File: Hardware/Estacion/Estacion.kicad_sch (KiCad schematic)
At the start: 13 parts, among them J1 Screw_Terminal_01x02, J2 Step_Down_Mini

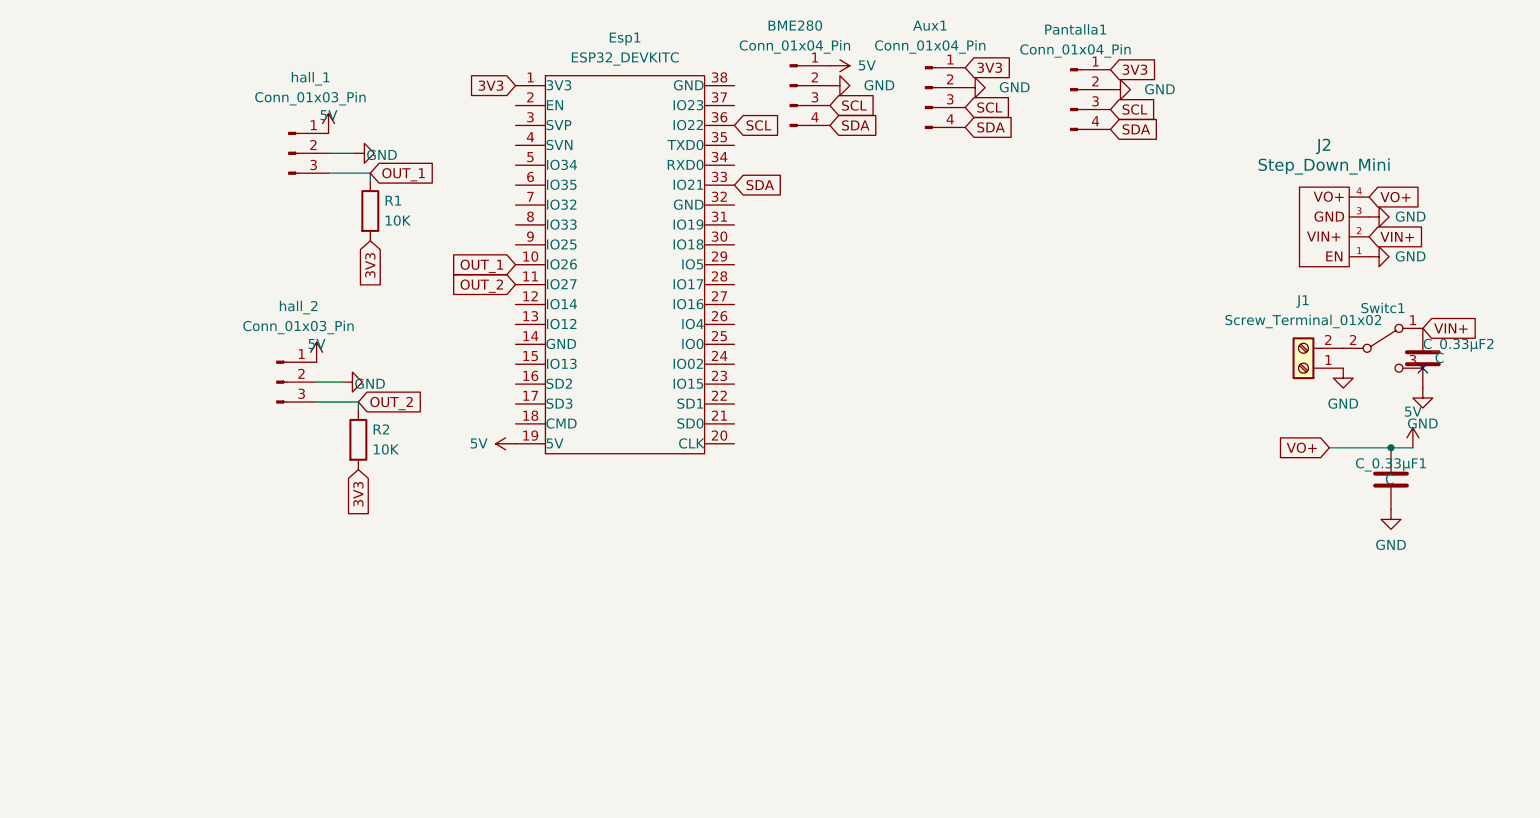
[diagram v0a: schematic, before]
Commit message: se avanzo el PCB y ESQUEMATICO
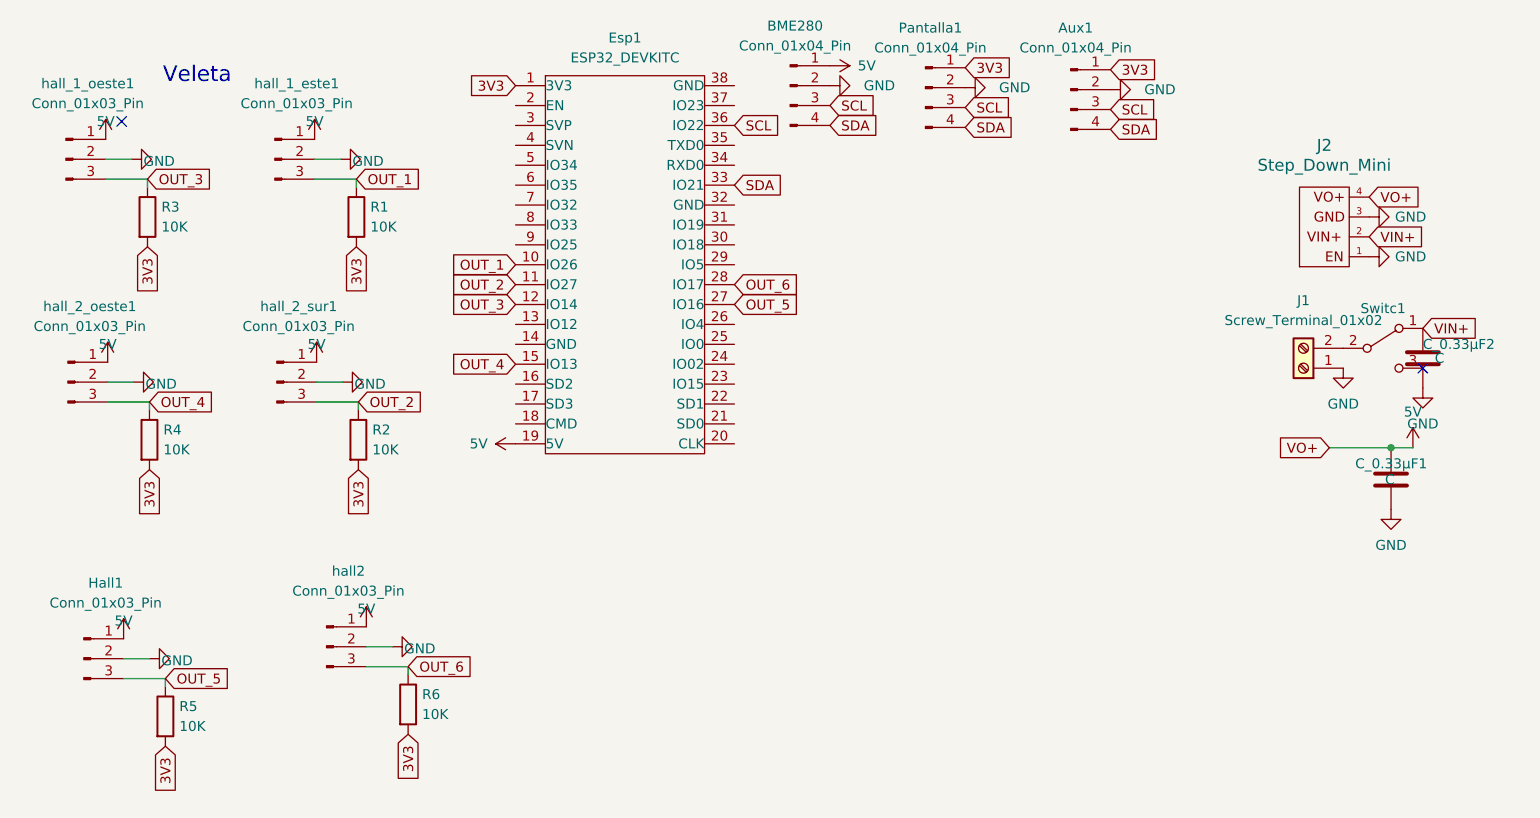
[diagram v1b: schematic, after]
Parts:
- added Hall1, hall2, hall_1_oeste1, hall_2_oeste1: Conn_01x03_Pin, Connector_JST:JST_PH_B3B-PH-K_1x03_P2.00mm_Vertical, symbol Connector:Conn_01x03_Pin
- added R3, R4, R5, R6: 10K, Resistor_SMD:R_0805_2012Metric_Pad1.20x1.40mm_HandSolder, symbol Device:R
- Aux1: renamed from Pantalla1; footprint Connector_PinSocket_2.54mm:PinSocket_1x04_P2.54mm_Vertical -> Connector_JST:JST_PH_B4B-PH-K_1x04_P2.00mm_Vertical
- BME280: footprint Connector_PinSocket_2.54mm:PinSocket_1x04_P2.54mm_Vertical -> Connector_JST:JST_PH_B4B-PH-K_1x04_P2.00mm_Vertical
- Pantalla1: renamed from Aux1; footprint Connector_PinSocket_2.54mm:PinSocket_1x04_P2.54mm_Vertical -> Connector_JST:JST_PH_B4B-PH-K_1x04_P2.00mm_Vertical
- R1, R2: footprint (none) -> Resistor_SMD:R_0805_2012Metric_Pad1.20x1.40mm_HandSolder
- hall_1_este1: renamed from hall_1; footprint Connector_PinHeader_2.54mm:PinHeader_1x03_P2.54mm_Vertical -> Connector_JST:JST_PH_B3B-PH-K_1x03_P2.00mm_Vertical
- hall_2_sur1: renamed from hall_2; footprint Connector_PinHeader_2.54mm:PinHeader_1x03_P2.54mm_Vertical -> Connector_JST:JST_PH_B3B-PH-K_1x03_P2.00mm_Vertical
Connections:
- net 3V3: now also R3.2, R4.2, R5.2, R6.2
- net 5V: now also Hall1.1 (Pin_1), hall2.1 (Pin_1), hall_1_oeste1.1 (Pin_1), hall_2_oeste1.1 (Pin_1)
- net GND: now also Hall1.2 (Pin_2), hall2.2 (Pin_2), hall_1_oeste1.2 (Pin_2), hall_2_oeste1.2 (Pin_2)
- net OUT_3: now reaches Esp1.12 (IO14)
- net OUT_3: now also R3.1, hall_1_oeste1.3 (Pin_3)
- net OUT_4: now reaches Esp1.15 (IO13)
- net OUT_4: now also R4.1, hall_2_oeste1.3 (Pin_3)
- net OUT_5: now reaches Esp1.27 (IO16)
- net OUT_5: now also Hall1.3 (Pin_3), R5.1
- net OUT_6: now reaches Esp1.28 (IO17)
- net OUT_6: now also R6.1, hall2.3 (Pin_3)
- no-connect marks 1 -> 2
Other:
- note added: "Veleta"
- moved on the sheet: R1, hall_1_este1

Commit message: Primera version del PCB
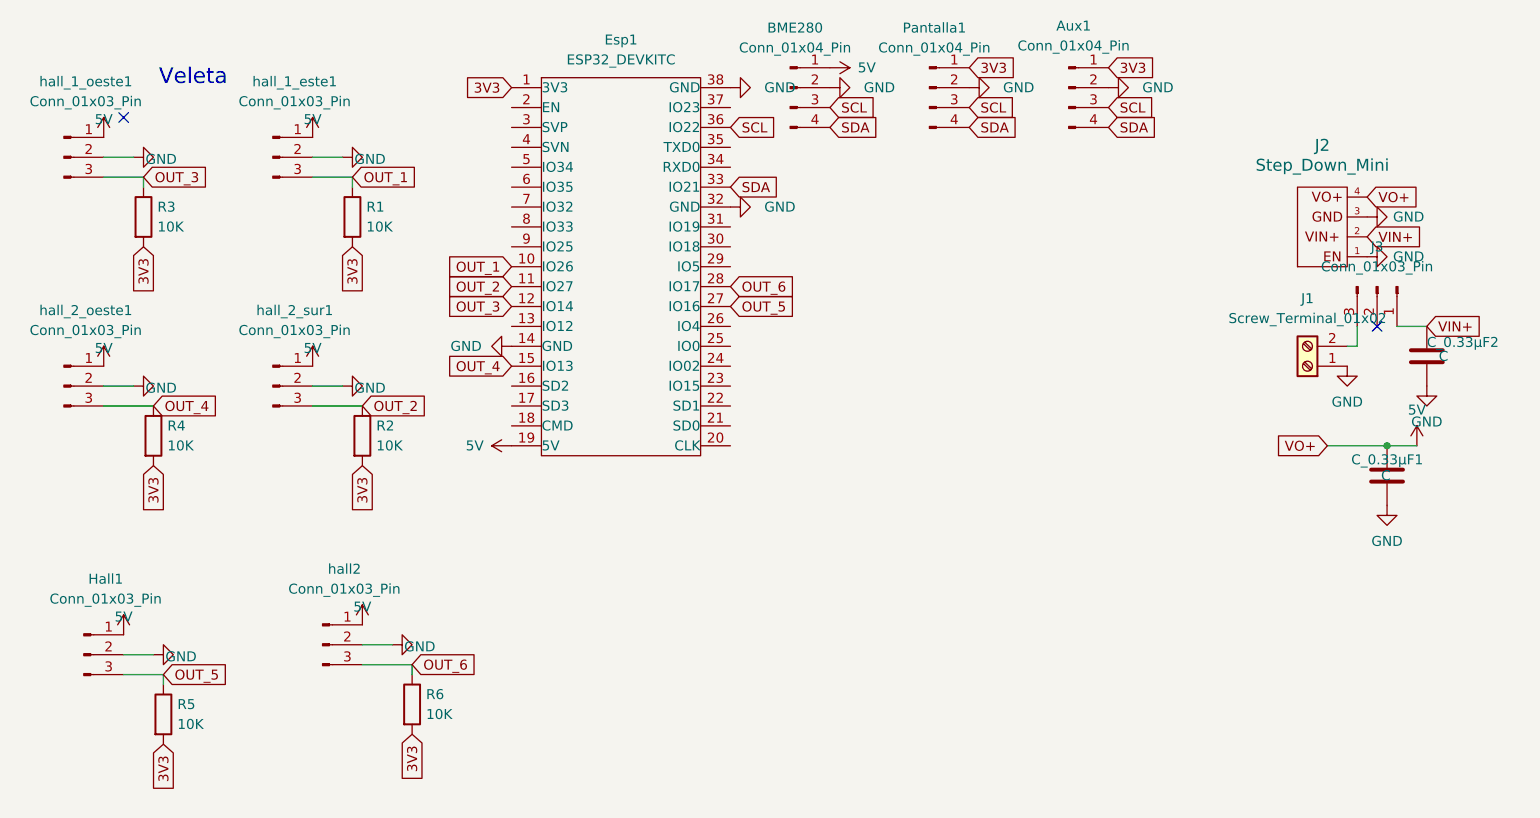
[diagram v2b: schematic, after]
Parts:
- removed Switc1: SW_SPDT, EESTN5:SW_SPDT_TH_100Mils_VERTICAL, symbol EESTN5:SW_SPDT
- added J3: Conn_01x03_Pin, Connector_JST:JST_PH_B3B-PH-K_1x03_P2.00mm_Vertical, symbol Connector:Conn_01x03_Pin
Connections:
- net GND: now also Esp1.14 (GND), Esp1.32 (GND), Esp1.38 (GND)
- net VIN+: now also J3.1 (Pin_1)
- net at J1.2 (Pin_2): now also J3.3 (Pin_3)
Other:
- moved on the sheet: C_0.33µF1, C_0.33µF2, Esp1, Hall1, J1, Pantalla1, R1, R2, R3, R4, R6, hall2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
